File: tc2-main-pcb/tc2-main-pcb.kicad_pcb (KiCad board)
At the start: 4 copper layers, 65 x 89 mm, 142 parts, among them J1 Screw_Terminal_01x01, J10 Conn_02x06_Odd_Even, J11 Conn_01x08, J2 Conn_01x03, J3 Conn_01x03, J4 Raspberry_Pi_2_3, J5 Screw_Terminal_01x01, J6 Screw_Terminal_01x01, J7 Screw_Terminal_01x01, J8 Screw_Terminal_01x01, J9 Conn_02x03_Odd_Even, Q1 Q_PMOS_GSD, SW2 K2-6639SP-M4SC-04, U1 ATtiny1616-M, U10 TD6810, U11 TD6810, U12 SIM7600G-H-M.2, U13 AHT21, U14 MAX98357AEWL+T, U15 74HC4052, U2 W25Q128JVS, U3 RP2040, U4 MT29F2G01ABAGDWB-IT, U6 PCF8563T, U7 ME6216A28XG, U8 Flir_LEPTON, U9 3N25000G33YC, Y1 Crystal_GND24, Y2 Crystal

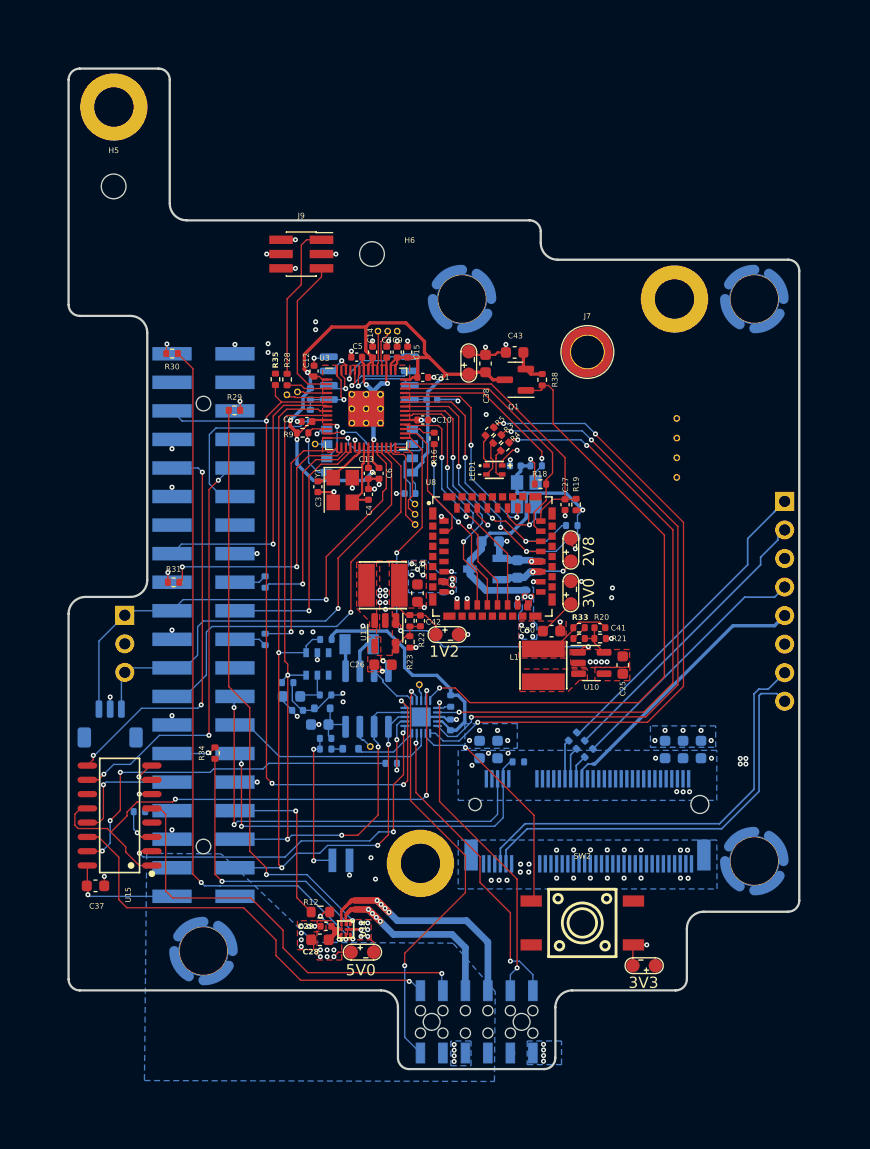
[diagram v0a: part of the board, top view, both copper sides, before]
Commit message: P3-Nov release
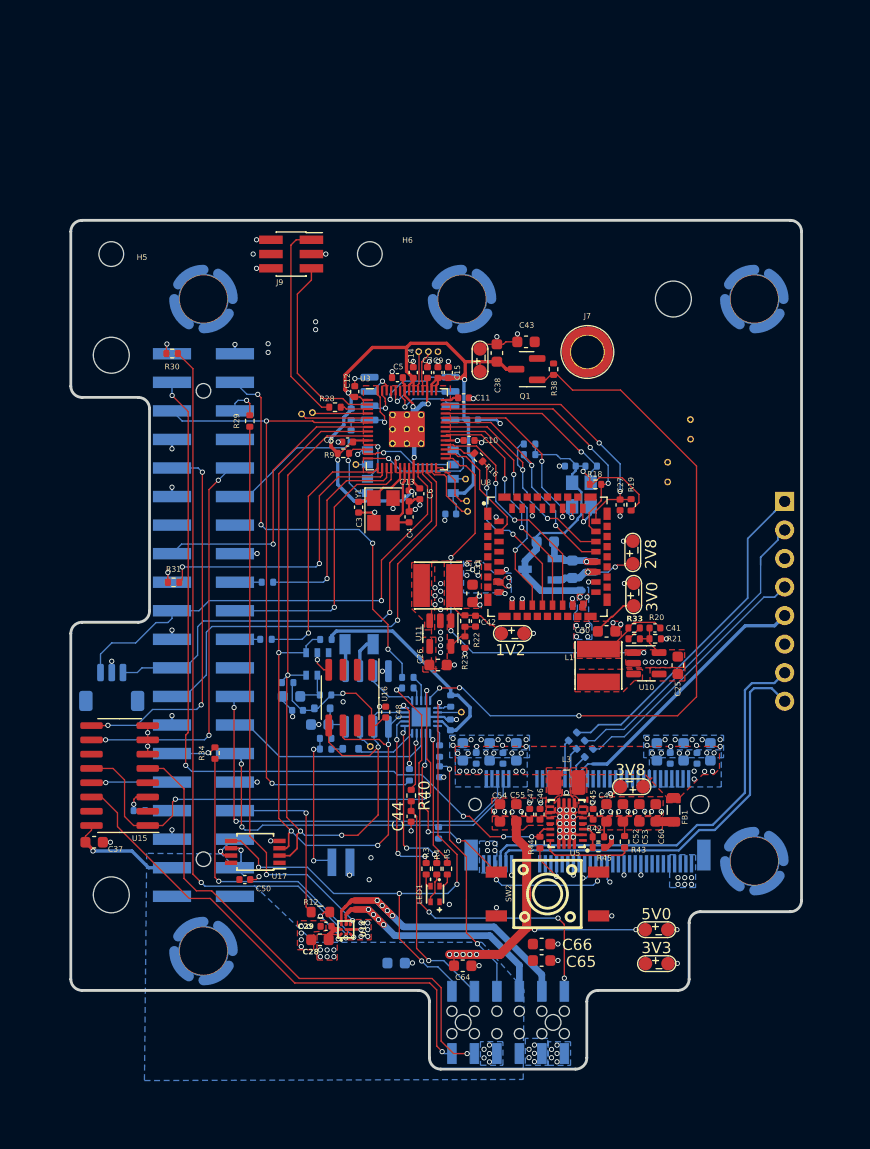
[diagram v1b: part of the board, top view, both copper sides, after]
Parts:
- removed TP24, TP25, TP28: TestPoint_2Pole, cacophony-library:test-point-2p
- added C40: 12pF, Capacitor_SMD:C_0402_1005Metric, B.Cu at (41.5, 11.8)
- added C44: 12pF, Capacitor_SMD:C_0402_1005Metric, F.Cu at (18.5, 17.0)
- added C45: 220nF, Capacitor_SMD:C_0402_1005Metric, F.Cu at (34.7, 16.8)
- added C46: 12pF, Capacitor_SMD:C_0402_1005Metric, F.Cu at (29.9, 16.8)
- added C47: 220nF, Capacitor_SMD:C_0402_1005Metric, F.Cu at (29.0, 16.8)
- added C48: 220nF, Capacitor_SMD:C_0402_1005Metric, F.Cu at (16.2, 7.74)
- added C49: 22uF, Capacitor_SMD:C_0603_1608Metric, F.Cu at (35.9, 16.7)
- added C50: 220nF, Capacitor_SMD:C_0402_1005Metric, F.Cu at (3.68, 22.6)
- added C51: 220nF, Capacitor_SMD:C_0402_1005Metric, B.Cu at (24.3, 11.8)
- added C52: 22uF, Capacitor_SMD:C_0603_1608Metric, F.Cu at (37.3, 16.7)
- added C53: 22uF, Capacitor_SMD:C_0603_1608Metric, F.Cu at (38.8, 16.7)
- added C54: 22uF, Capacitor_SMD:C_0603_1608Metric, F.Cu at (26.4, 16.7)
- added C55: 22uF, Capacitor_SMD:C_0603_1608Metric, F.Cu at (27.8, 16.7)
- added C56: 12pF, Capacitor_SMD:C_0402_1005Metric, B.Cu at (21.0, 13.1)
- added C57: 22uF, Capacitor_SMD:C_0603_1608Metric, B.Cu at (27.8, 11.3)
- added C58: 22uF, Capacitor_SMD:C_0603_1608Metric, B.Cu at (25.4, 11.3)
- added C59: 22uF, Capacitor_SMD:C_0603_1608Metric, B.Cu at (23.1, 11.3)
- added C60: 22uF, Capacitor_SMD:C_0603_1608Metric, F.Cu at (40.2, 16.7)
- added C62: 22uF, Capacitor_SMD:C_0603_1608Metric, B.Cu at (17.1, 30.1)
- added C64: 22uF, Capacitor_SMD:C_0603_1608Metric, F.Cu at (23.1, 30.3)
- added C65: 22uF, Capacitor_SMD:C_0603_1608Metric, F.Cu at (30.1, 29.8)
- added C66: 22uF, Capacitor_SMD:C_0603_1608Metric, F.Cu at (30.1, 28.4)
- added FB1: FerriteBead, Inductor_SMD:L_0805_2012Metric, F.Cu at (41.8, 16.4)
- added L3: INDUCTOR, Inductor_SMD:L_1008_2520Metric, F.Cu at (32.3, 14.0)
- added R40: 10k, Resistor_SMD:R_0402_1005Metric, F.Cu at (18.5, 15.2)
- added R42: 1M, Resistor_SMD:R_0402_1005Metric, F.Cu at (35.1, 18.8)
- added R43: 1M, Resistor_SMD:R_0402_1005Metric, F.Cu at (37.5, 19.3)
- added R44: 100k, Resistor_SMD:R_0402_1005Metric, F.Cu at (29.9, 19.3)
- added R45: 150k, Resistor_SMD:R_0402_1005Metric, F.Cu at (35.1, 19.8)
- added R46: 1k, Resistor_SMD:R_0402_1005Metric, B.Cu at (18.2, 5.60)
- added R49: 10k, Resistor_SMD:R_0402_1005Metric, B.Cu at (21.0, 11.2)
- added TP10: TP_2P, cacophony-library:test-point-2p, F.Cu at (40.3, 27.1)
- added TP2: TestPoint, cacophony-library:TP, F.Cu at (22.9, 7.75)
- added TP3: TP_2P, cacophony-library:test-point-2p, F.Cu at (24.6, -23.6)
- added TP5: TP_2P, cacophony-library:test-point-2p, F.Cu at (38.2, -6.46)
- added U16: M24C02-WMN, Package_SO:SOIC-8_3.9x4.9mm_P1.27mm, F.Cu at (13.0, 6.46)
- added U17: PCA9515ADP,118, Package_SO:TSSOP-8_3x3mm_P0.65mm, F.Cu at (4.61, 20.2)
- added U5: TPS6302x, cacophony-library:VSON-14_L4.0-W3.0-P0.50-BL-EP_TI_DSJ, F.Cu at (32.3, 17.7)
- C32: value 10uF -> 12pF; footprint Capacitor_SMD:C_0603_1608Metric -> Capacitor_SMD:C_0402_1005Metric
- C33, C34, C35: value 10uF -> 22uF
- C36: value 10uF -> 220nF; footprint Capacitor_SMD:C_0603_1608Metric -> Capacitor_SMD:C_0402_1005Metric
- H1, H3, H4: footprint cacophony-library:Mouning_Hole_M3 -> cacophony-library:MountingHole_3.2mm_M3
- J2: value Conn_01x03 -> Screw_Terminal_01x01; footprint Connector_PinHeader_2.54mm:PinHeader_1x03_P2.54mm_Vertical -> cacophony-library:SMTSO25
- J4: footprint cacophony-library:RPI_HDR-SMD_40P-P2.54-V-F-R2-C20-S8.7-EH -> cacophony-library:HDR-SMD_40P-P2.54-V-F-R2-C20-LS8.2-EH
- J7: footprint cacophony-library:SMD_BD4.4-L4.4-D2.8 -> cacophony-library:M2_modem_mount_screw
- R15: value 100k -> 1k
- R35: value 100k -> 1k; moved to B.Cu
- TP1: value TestPoint -> TP_2P; footprint cacophony-library:TP -> cacophony-library:test-point-2p
- TP4, TP6, TP8: value TestPoint_2Pole -> TP_2P
- U15: footprint cacophony-library:SOP-16_L10.0-W3.9-P1.27-LS6.0-BL -> Package_SO:SOP-16_3.9x9.9mm_P1.27mm
- moved TP6 56.0 mm to (40.3, 30.1), turned to 180 degrees
- moved R5 39.1 mm to (21.7, 21.7), turned to -90 degrees
- moved R3 38.7 mm to (19.8, 21.7), turned to -90 degrees
- moved LED1 38.1 mm to (20.6, 23.9), turned to -90 degrees
- moved R4 38.0 mm to (20.8, 21.7), turned to -90 degrees
- moved R35 29.0 mm to (18.2, 4.66), turned to 180 degrees
- moved J2 29.0 mm to (0.00, -29.0)
- moved H3 27.6 mm to (-8.20, 24.0)
- moved H4 22.1 mm to (-8.20, -24.0)
- moved TP1 21.0 mm to (38.1, 14.4)
- moved C33 18.9 mm to (45.1, 11.3)
- moved R24 9.50 mm to (20.9, 18.5), turned to 90 degrees
- moved R36 8.25 mm to (29.0, -15.2)
- moved R13 8.16 mm to (29.0, -16.1)
- moved H5 6.02 mm to (-8.20, -33.0)
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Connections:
- net /PDM_CLOCK_ renamed /PDM_CLOCK_PHY
- net LED_B renamed ~{LED_B}
- net LED_G renamed ~{LED_G}
- net LED_R renamed ~{LED_R}
- net Net-(BT1-+) renamed /RTC_BATTERY
- net Net-(D3-K) renamed /RTC_VDD
- net Net-(U1-PA5) renamed /ATtiny1616/~{LED_R_PHY}
- net Net-(U13-VDD) renamed /AHT21_VDD
- net Net-(U4-~{HOLD}/IO3) renamed /MEM_~{HOLD}/IO3
- net Net-(U4-~{WP}/IO2) renamed /MEM_~{WP}/IO2
- net Net-(U6-CLKO) renamed /RTC_CLKO
- net Net-(U6-OSCI) renamed /RTC_OSCI
- net Net-(U6-OSCO) renamed /RTC_OSCO
- net RTC_BT_SENSE renamed RTC_BT_SENSE_PHY
- C32 pad 1: +3V3 -> GND
- C32 pad 2: GND -> +3V8
- C33 pad 1: +3V3 -> +3V8
- C34 pad 1: +3V3 -> +3V8
- C35 pad 1: +3V3 -> +3V8
- C36 pad 1: +3V3 -> GND
- C36 pad 2: GND -> +3V8
- J10 pad 1: GND -> 5V_EN
- J10 pad 10: OUT_TX -> +3V3
- J10 pad 12: OUT_RX -> GND
- J10 pad 2: BATT_SENSE -> OUT_RX
- J10 pad 3: +3V3 -> BATT_SENSE_HV
- J10 pad 4: 5V_EN -> OUT_TX
- J10 pad 5: +5V -> BATT_SENSE_LV
- J10 pad 6: SPEAKER_+ -> GND
- J10 pad 7: GND -> SPEAKER_-
- J10 pad 8: SPEAKER_- -> +5V
- J10 pad 9: unconnected-(J10-Pin_9-Pad9) -> SPEAKER_+
- J2 pad 1: SW_CLK -> unconnected-(J2-Pin_1-Pad1)
- J4 pad 13: ~{PI_SHUTDOWN} -> ~{PI_POWERED_OFF}
- J4 pad 3: SDA -> RPI_SDA
- J4 pad 36: ~{WAKEUP_PING} -> ~{READ_ATTINY_CMD_REG}
- J4 pad 37: unconnected-(J4-GPIO26-Pad37) -> ~{PI_SHUTDOWN}
- J4 pad 38: unconnected-(J4-GPIO20/MOSI1-Pad38) -> MODEM_POWER_EN
- J4 pad 5: SCL -> RPI_SCL
- R15 pad 1: ATTINY_TX -> /ATtiny1616/~{READ_ATTINY_CMD_REG_PHY}
- R15 pad 2: Net-(U1-PB2) -> ~{READ_ATTINY_CMD_REG}
- R3 pad 1: Net-(U1-PA4) -> /ATtiny1616/~{LED_G_PHY}
- R35 pad 1: +3V3 -> /ATtiny1616/~{PI_SHUTDOWN_PHY}
- R35 pad 2: ~{WAKEUP_PING} -> ~{PI_SHUTDOWN}
- R4 pad 1: Net-(U1-PA3) -> /ATtiny1616/~{LED_B_PHY}
- SW2 pad 1: Net-(U1-PA6) -> /ATtiny1616/ATtiny_SW
- SW2 pad 2: unconnected-(SW2-Pad2) -> /ATtiny1616/ATtiny_SW
- SW2 pad 3: unconnected-(SW2-Pad3) -> GND
- TP1 pad 1: Net-(U1-PC3) -> GND
- TP6 pad 2: +3V3_rp2040 -> +3V3
- U1 pad 11: ATTINY_RX -> /ATtiny1616/~{LED_B_PHY}
- U1 pad 12: Net-(U1-PB2) -> /ATtiny1616/~{LED_G_PHY}
- U1 pad 15: ~{WAKEUP_PING} -> /ATtiny1616/~{READ_ATTINY_CMD_REG_PHY}
- U1 pad 17: EN_PERIPH_POWER -> /ATtiny1616/EN_PERIPH_POWER_PHY
- U1 pad 18: Net-(U1-PC3) -> /ATtiny1616/~{PI_SHUTDOWN_PHY}
- U1 pad 2: Net-(U1-PA3) -> /ATtiny1616/ATTINY_PA3
- U1 pad 5: Net-(U1-PA4) -> BATT_SENSE_LOW_VOLTAGE_PHY
- U1 pad 7: Net-(U1-PA6) -> /ATtiny1616/ATtiny_SW
- U1 pad 8: ~{PI_SHUTDOWN} -> ~{PI_POWERED_OFF}
- U1 pad 9: BATT_SENSE -> BATT_SENSE_HIGH_VOLTAGE_PHY
- U12 pad 2: +3V3 -> +3V8
- U12 pad 4: +3V3 -> +3V8
- U12 pad 70: +3V3 -> +3V8
- U12 pad 72: +3V3 -> +3V8
- U12 pad 74: +3V3 -> +3V8
- U15 pad 15: ATTINY_TX -> unconnected-(U15-1Y2-Pad15)
- U15 pad 2: ATTINY_RX -> unconnected-(U15-2Y2-Pad2)
- U3 pad 6: ~{WAKEUP_PING} -> ~{READ_ATTINY_CMD_REG}
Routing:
- net MODEM_POWER_EN: track 0.00 -> 70.3 mm, vias 0 -> 5
- net ~{WAKEUP_PING}: track 69.6 -> 0.00 mm, vias 4 -> 0
- net ~{READ_ATTINY_CMD_REG}: track 0.00 -> 62.7 mm, vias 0 -> 2
- net Net-(U1-PA4): track 57.4 -> 0.00 mm, vias 3 -> 0
- net Net-(U1-PA3): track 53.7 -> 0.00 mm, vias 3 -> 0
- net /ATtiny1616/~{LED_R_PHY}: track 60.1 -> 12.2 mm, vias 3 -> 1
- net ATTINY_RX: track 34.7 -> 0.00 mm, vias 3 -> 0
- net ATTINY_TX: track 32.9 -> 0.00 mm, vias 3 -> 0
- net +5V: track 13.9 -> 41.9 mm, vias 7 -> 14
- net BATT_SENSE: track 27.7 -> 0.00 mm, vias 2 -> 0
- net /ATtiny1616/ATtiny_SW: track 0.00 -> 27.5 mm, vias 0 -> 5
- net BATT_SENSE_LV: track 0.00 -> 23.4 mm, vias 0 -> 2
- net 5V_EN: track 30.5 -> 52.7 mm, vias 2 -> 5
- net Net-(U1-PA6): track 20.2 -> 0.00 mm, vias 1 -> 0
- net BATT_SENSE_HV: track 0.00 -> 20.0 mm, vias 0 -> 1
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- added copper zone on B.Cu, net +3V8
- added copper zone on F.Cu, net +3V8
- added copper zone on F.Cu, net /modem/3V3_L1
- added copper zone on F.Cu, net /modem/3V3_L2
- added copper zone on F.Cu, net /modem/MODEM_3V8
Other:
- board size 65 x 89 mm -> 65 x 75.5 mm
- board text added: "3V8"
- board text removed: "CLK"
- board text removed: "GND"
- board text removed: "SWD"
